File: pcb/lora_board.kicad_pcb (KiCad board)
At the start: 2 copper layers, 20 x 45 mm, 32 parts, among them J1 USB_C_Receptacle_USB2.0_16P, J2 Conn_01x02_Shielded, J3 Conn_01x05, J4 Qi Charger, Q1 AO3400A, SW1 SW_Push, SW2 SW_SPDT, U1 E73-2G4M08S1C, U2 AP2112K-3.3, U3 E22-900MM22S, U4 MCP73831-2-OT

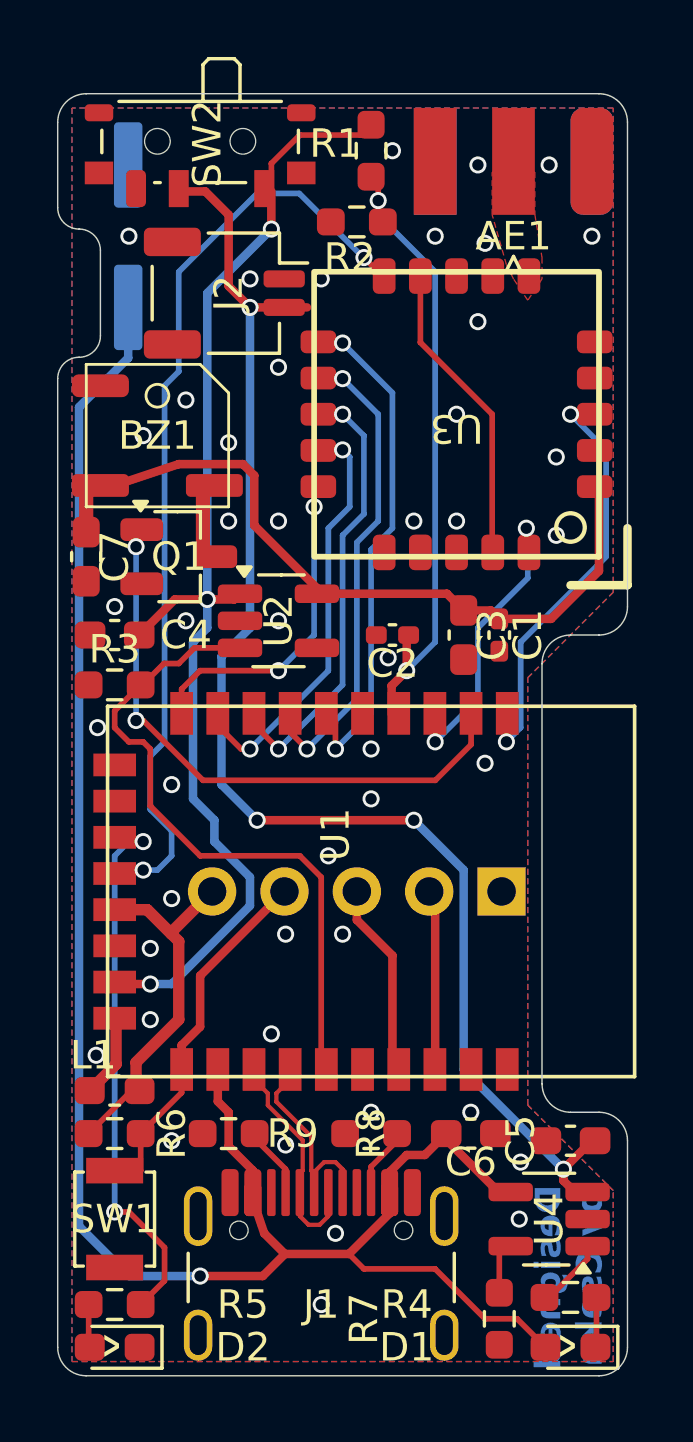
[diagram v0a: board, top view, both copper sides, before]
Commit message: v2 rc3
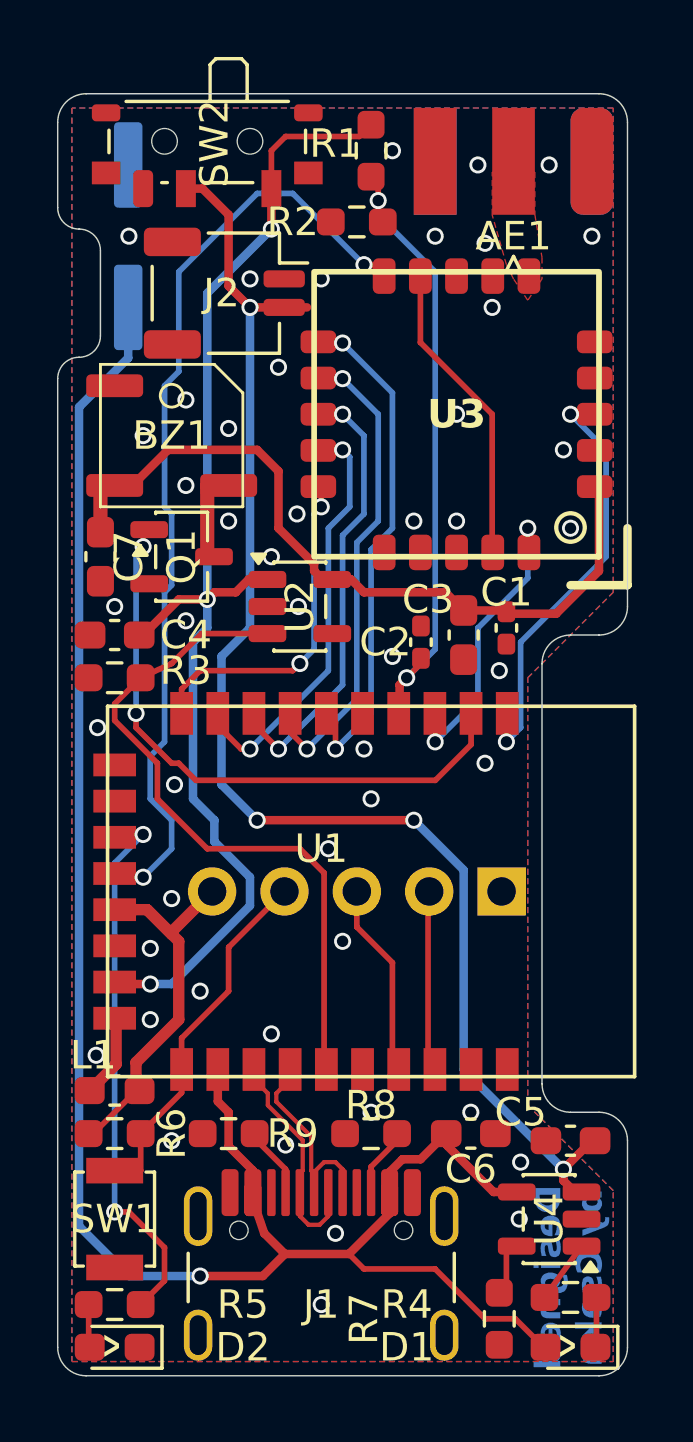
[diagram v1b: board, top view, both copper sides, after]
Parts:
- Q1: footprint Package_TO_SOT_SMD:SOT-23_Handsoldering -> Package_TO_SOT_SMD:SOT-23-3
- U2, U4: footprint Package_TO_SOT_SMD:SOT-23-5_HandSoldering -> Package_TO_SOT_SMD:SOT-23-5
- moved C2 1.03 mm to (107.8, 94.2), turned to 90 degrees
- moved U2 0.90 mm to (103.5, 93.0)
- moved BZ1 0.50 mm to (99.0, 87.0)
- moved C7 0.50 mm to (96.5, 91.2)
- moved C1 0.35 mm to (110.8, 93.8)
- moved R3 0.25 mm to (97.0, 95.5)
- moved SW2 0.25 mm to (100.2, 77.0)
- moved Q1 0.10 mm to (99.3, 91.2)
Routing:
- net VCC: track 42.1 -> 43.6 mm
- net /REG_EN: track 23.3 -> 24.1 mm
- net /BAT_SENSE: track 22.9 -> 22.2 mm
- net GND: vias 46 -> 49
